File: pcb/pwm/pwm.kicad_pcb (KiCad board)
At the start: 2 copper layers, 145 x 145 mm, 19 parts, among them Q1 IRFB4321PBF, Q2 IRFB4321PBF, Q3 IRFB4321PBF, Q4 IRFB4321PBF, Q5 IRFB4321PBF, Q6 IRFB4321PBF, Q7 IRFB4321PBF, Q8 IRFB4321PBF, U1 pwm_meson0, X1 Conn_01x04_Male, X2 Conn_01x04_Male, X3 Conn_01x02_Male, X4 Conn_01x02_Male

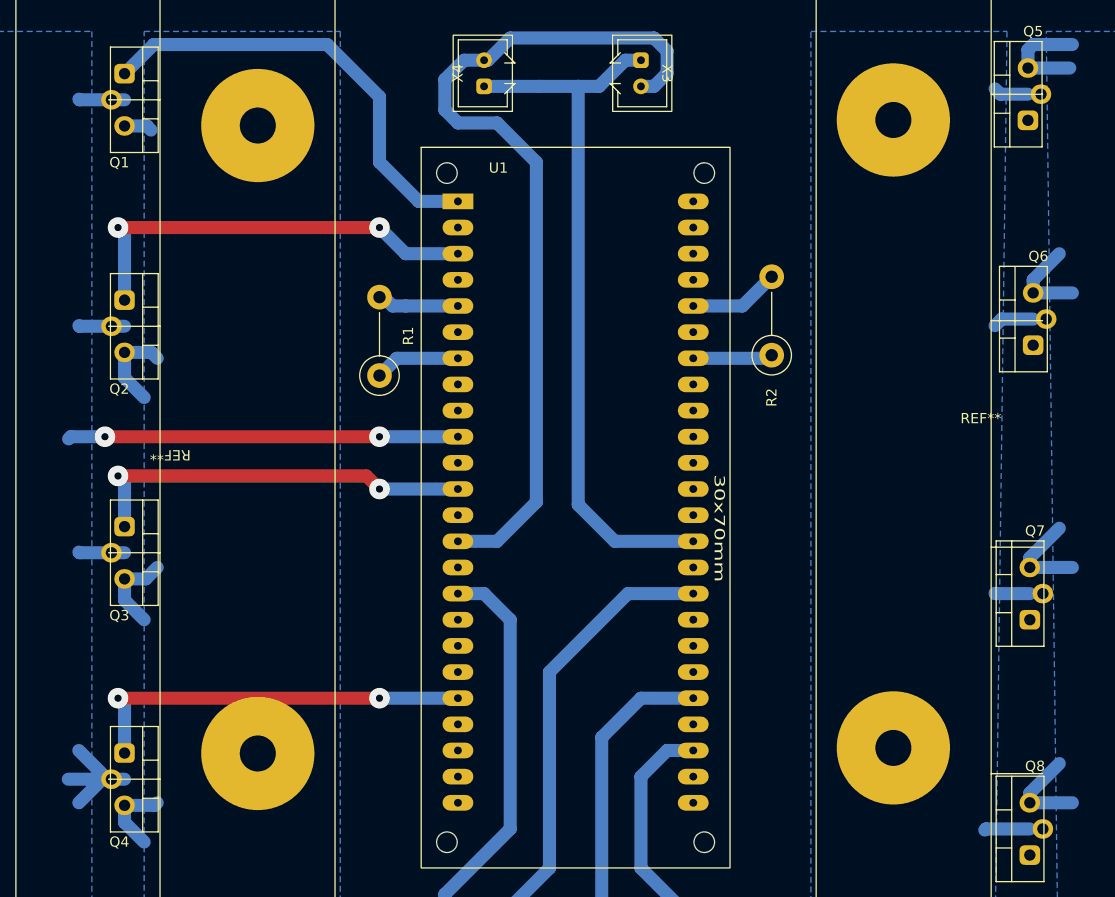
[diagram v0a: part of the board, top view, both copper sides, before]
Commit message: Signed-off-by: Dmitry Ponyatov <dponyatov@samsa.local>
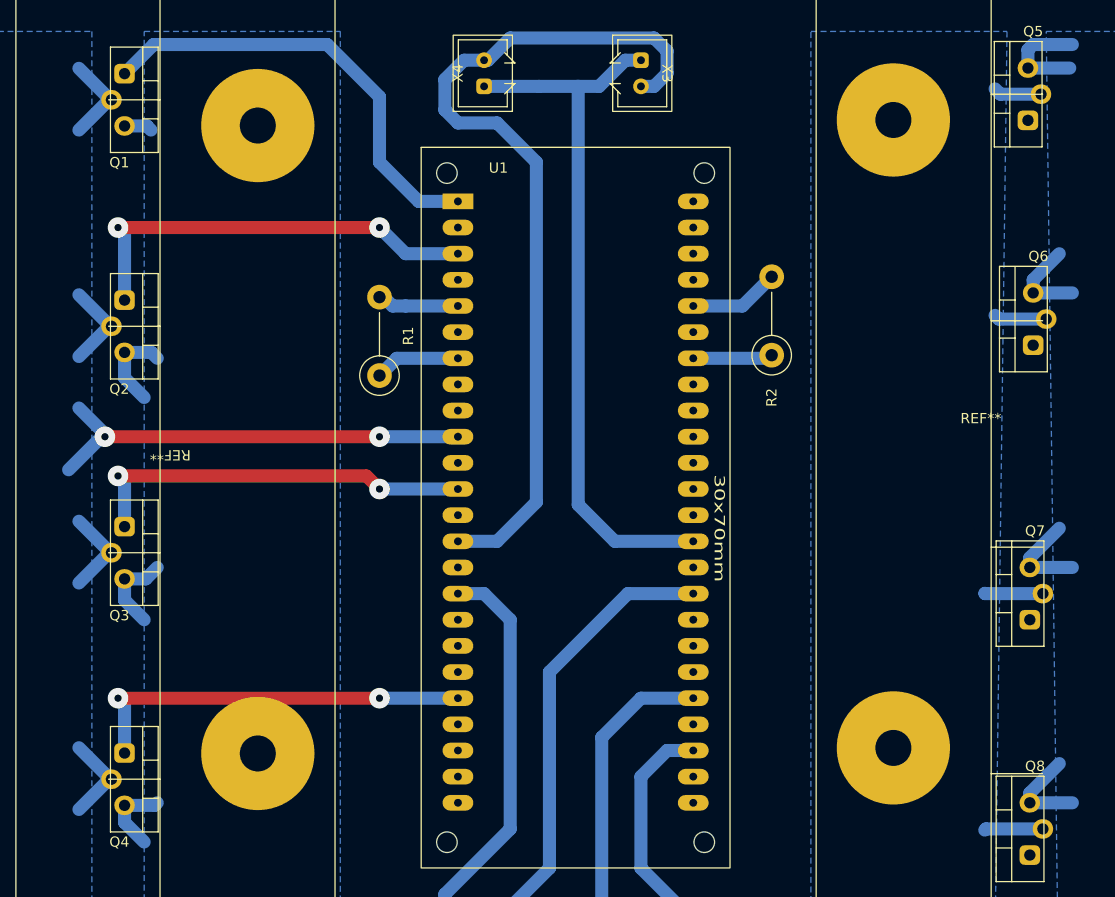
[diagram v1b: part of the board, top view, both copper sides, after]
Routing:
- net /+60V: track 66.1 -> 78.6 mm
- net /phase: track 42.8 -> 48.7 mm
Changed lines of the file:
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@@
   (segment (start 76.2 97.79) (end 49.53 97.79) (width 1.27) (layer "F.Cu") (net 2))
   (segment (start 50.165 131.06) (end 49.78 131.06) (width 1.27) (layer "B.Cu") (net 2))
-  (segment (start 47 65) (end 47.06 65.06) (width 1.27) (layer "B.Cu") (net 2))
-  (segment (start 46 98) (end 46.21 97.79) (width 1.27) (layer "B.Cu") (net 2))
-  (segment (start 50.165 131.06) (end 49.28 131.06) (width 1.27) (layer "B.Cu") (net 2))
+  (segment (start 50.06 87.06) (end 47 84) (width 1.27) (layer "B.Cu") (net 2))
+  (segment (start 49.53 97.79) (end 49.21 97.79) (width 1.27) (layer "B.Cu") (net 2))
+  (segment (start 49.53 97.53) (end 47 95) (width 1.27) (layer "B.Cu") (net 2))
+  (segment (start 50.165 87.06) (end 49.94 87.06) (width 1.27) (layer "B.Cu") (net 2))
+  (segment (start 50.165 65.06) (end 50.06 65.06) (width 1.27) (layer "B.Cu") (net 2))
   (segment (start 83.82 97.79) (end 76.2 97.79) (width 1.27) (layer "B.Cu") (net 2))
-  (segment (start 47.06 109.06) (end 47 109) (width 1.27) (layer "B.Cu") (net 2))
-  (segment (start 49.53 97.79) (end 46.21 97.79) (width 1.27) (layer "B.Cu") (net 2))
-  (segment (start 51.435 131.06) (end 49.28 131.06) (width 1.27) (layer "B.Cu") (net 2))
-  (segment (start 51.435 109.06) (end 47.06 109.06) (width 1.27) (layer "B.Cu") (net 2))
-  (segment (start 51.435 65.06) (end 47.06 65.06) (width 1.27) (layer "B.Cu") (net 2))
-  (segment (start 47 87) (end 47.06 87.06) (width 1.27) (layer "B.Cu") (net 2))
-  (segment (start 49.28 131.06) (end 46.99 133.35) (width 1.27) (layer "B.Cu") (net 2))
-  (segment (start 49.78 131.06) (end 46.99 128.27) (width 1.27) (layer "B.Cu") (net 2))
-  (segment (start 51.435 87.06) (end 47.06 87.06) (width 1.27) (layer "B.Cu") (net 2))
-  (segment (start 50.165 131.06) (end 45.97 131.06) (width 1.27) (layer "B.Cu") (net 2))
+  (segment (start 49.53 97.79) (end 49.53 97.53) (width 1.27) (layer "B.Cu") (net 2))
+  (segment (start 50.165 109.06) (end 50.06 109.06) (width 1.27) (layer "B.Cu") (net 2))
+  (segment (start 50.165 109.06) (end 49.94 109.06) (width 1.27) (layer "B.Cu") (net 2))
+  (segment (start 50.165 131.06) (end 50.06 131.06) (width 1.27) (layer "B.Cu") (net 2))
+  (segment (start 50.165 131.06) (end 49.94 131.06) (width 1.27) (layer "B.Cu") (net 2))
+  (segment (start 50.165 65.06) (end 49.94 65.06) (width 1.27) (layer "B.Cu") (net 2))
+  (segment (start 49.94 65.06) (end 47 68) (width 1.27) (layer "B.Cu") (net 2))
+  (segment (start 50.06 131.06) (end 47 128) (width 1.27) (layer "B.Cu") (net 2))
+  (segment (start 50.165 87.06) (end 50.06 87.06) (width 1.27) (layer "B.Cu") (net 2))
+  (segment (start 49.21 97.79) (end 46 101) (width 1.27) (layer "B.Cu") (net 2))
+  (segment (start 50.06 65.06) (end 47 62) (width 1.27) (layer "B.Cu") (net 2))
+  (segment (start 49.94 87.06) (end 47 90) (width 1.27) (layer "B.Cu") (net 2))
+  (segment (start 49.94 109.06) (end 47 112) (width 1.27) (layer "B.Cu") (net 2))
+  (segment (start 49.94 131.06) (end 47 134) (width 1.27) (layer "B.Cu") (net 2))
+  (segment (start 50.06 109.06) (end 47 106) (width 1.27) (layer "B.Cu") (net 2))
   (segment (start 54.36 133.6) (end 54.61 133.35) (width 1.27) (layer "B.Cu") (net 3))
-  (segment (start 139.192 64.516) (end 136.516 64.516) (width 1.27) (layer "B.Cu") (net 3))
   (segment (start 51.435 92.075) (end 53.34 93.98) (width 1.27) (layer "B.Cu") (net 3))
   (segment (start 51.435 89.6) (end 51.435 92.075) (width 1.27) (layer "B.Cu") (net 3))
   (segment (start 54.61 90.17) (end 54.04 89.6) (width 1.27) (layer "B.Cu") (net 3))
-  (segment (start 139.7 86.36) (end 136.64 86.36) (width 1.27) (layer "B.Cu") (net 3))
   (segment (start 51.435 89.6) (end 54.04 89.6) (width 1.27) (layer "B.Cu") (net 3))
+  (segment (start 140.645 135.89) (end 135.11 135.89) (width 1.27) (layer "B.Cu") (net 3))
   (segment (start 51.435 111.6) (end 51.470407 111.6) (width 1.27) (layer "B.Cu") (net 3))
   (segment (start 51.435 111.6) (end 53.5 111.6) (width 1.27) (layer "B.Cu") (net 3))
+  (segment (start 140.97 86.36) (end 136.36 86.36) (width 1.27) (layer "B.Cu") (net 3))
   (segment (start 51.435 133.6) (end 54.36 133.6) (width 1.27) (layer "B.Cu") (net 3))
-  (segment (start 136.516 64.516) (end 136 64) (width 1.27) (layer "B.Cu") (net 3))
+  (segment (start 140.462 64.516) (end 136.516 64.516) (width 1.27) (layer "B.Cu") (net 3))
   (segment (start 51.435 67.6) (end 53.6 67.6) (width 1.27) (layer "B.Cu") (net 3))
+  (segment (start 135 136) (end 135.11 135.89) (width 1.27) (layer "B.Cu") (net 3))
   (segment (start 51.435 113.665) (end 53.34 115.57) (width 1.27) (layer "B.Cu") (net 3))
-  (segment (start 139.375 135.89) (end 135.11 135.89) (width 1.27) (layer "B.Cu") (net 3))
+  (segment (start 135 113) (end 135.03 113.03) (width 1.27) (layer "B.Cu") (net 3))
   (segment (start 51.435 133.6) (end 51.435 135.255) (width 1.27) (layer "B.Cu") (net 3))
   (segment (start 51.435 111.6) (end 51.435 113.665) (width 1.27) (layer "B.Cu") (net 3))
   (segment (start 51.435 135.255) (end 53.34 137.16) (width 1.27) (layer "B.Cu") (net 3))
-  (segment (start 139.375 113.03) (end 136.03 113.03) (width 1.27) (layer "B.Cu") (net 3))
-  (segment (start 136.03 113.03) (end 136 113) (width 1.27) (layer "B.Cu") (net 3))
+  (segment (start 136.516 64.516) (end 136 64) (width 1.27) (layer "B.Cu") (net 3))
   (segment (start 53.6 67.6) (end 54 68) (width 1.27) (layer "B.Cu") (net 3))
+  (segment (start 140.645 113.03) (end 135.03 113.03) (width 1.27) (layer "B.Cu") (net 3))
   (segment (start 53.5 111.6) (end 54.61 110.49) (width 1.27) (layer "B.Cu") (net 3))
-  (segment (start 136.64 86.36) (end 136 87) (width 1.27) (layer "B.Cu") (net 3))
-  (segment (start 135 136) (end 135.11 135.89) (width 1.27) (layer "B.Cu") (net 3))
   (segment (start 51.470407 111.6) (end 51.630407 111.76) (width 1.27) (layer "B.Cu") (net 3))
+  (segment (start 136 86) (end 136.36 86.36) (width 1.27) (layer "B.Cu") (net 3))
   (segment (start 76.2 77.47) (end 50.8 77.47) (width 1.27) (layer "F.Cu") (net 4))
   (segment (start 51.435 84.52) (end 51.435 78.105) (width 1.27) (layer "B.Cu") (net 4))
